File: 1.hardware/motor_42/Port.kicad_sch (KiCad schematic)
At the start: 17 parts, among them J1 PC_CONN, J11 WAGO_2060, J12 WAGO_2060, J2 MT6816_CONN, J4 DEBUG, J5 CAN_IN, J6 CAN_OUT, J7 ESP_DOWNLOAD, J9 WS2812_OUT, U3 SN65HVD232

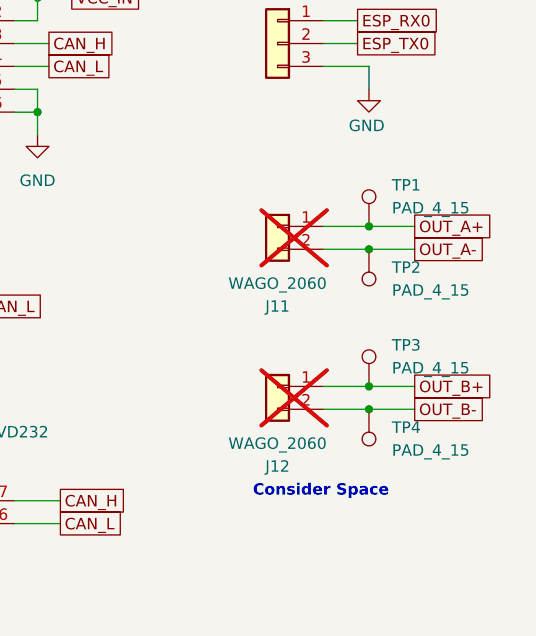
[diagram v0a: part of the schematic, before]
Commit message: 중간 저장
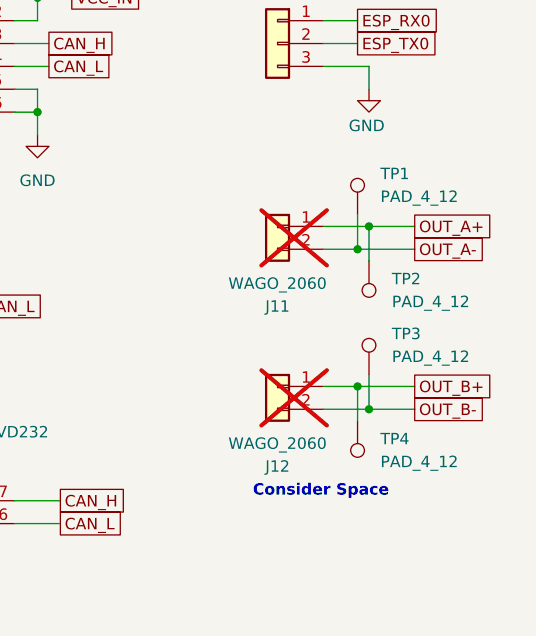
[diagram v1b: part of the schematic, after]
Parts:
- TP1, TP2, TP3, TP4: value PAD_4_15 -> PAD_4_12; footprint New_Footprints:custom_pad_4_15 -> New_Footprints:custom_pad_2_5
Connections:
- net OUT_A+: now also TP2.1; no longer TP1.1
- net OUT_A-: now also TP1.1; no longer TP2.1
- net OUT_B+: now also TP4.1; no longer TP3.1
- net OUT_B-: now also TP3.1; no longer TP4.1
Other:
- moved on the sheet: TP1, TP2, TP3, TP4
